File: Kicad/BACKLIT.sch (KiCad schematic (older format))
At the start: 88 parts, among them U1 PAM2804

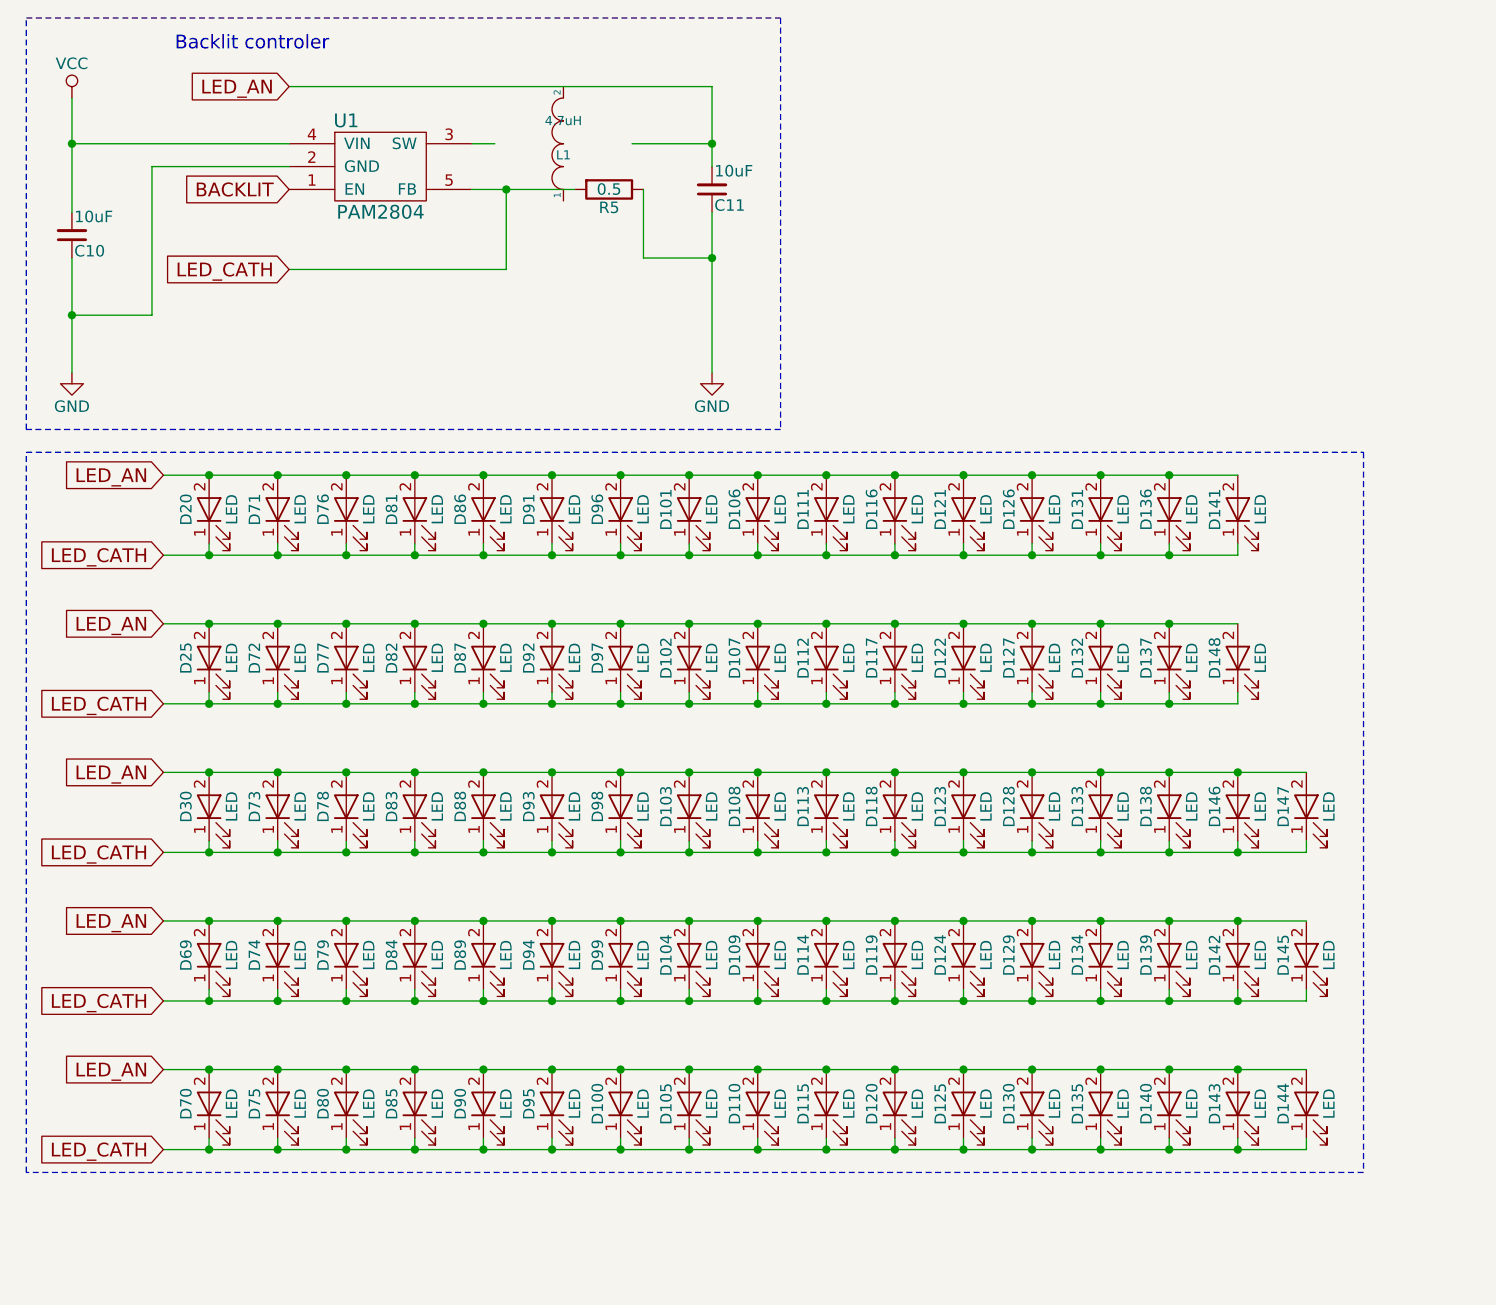
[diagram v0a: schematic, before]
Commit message: - First draw for Rev. B
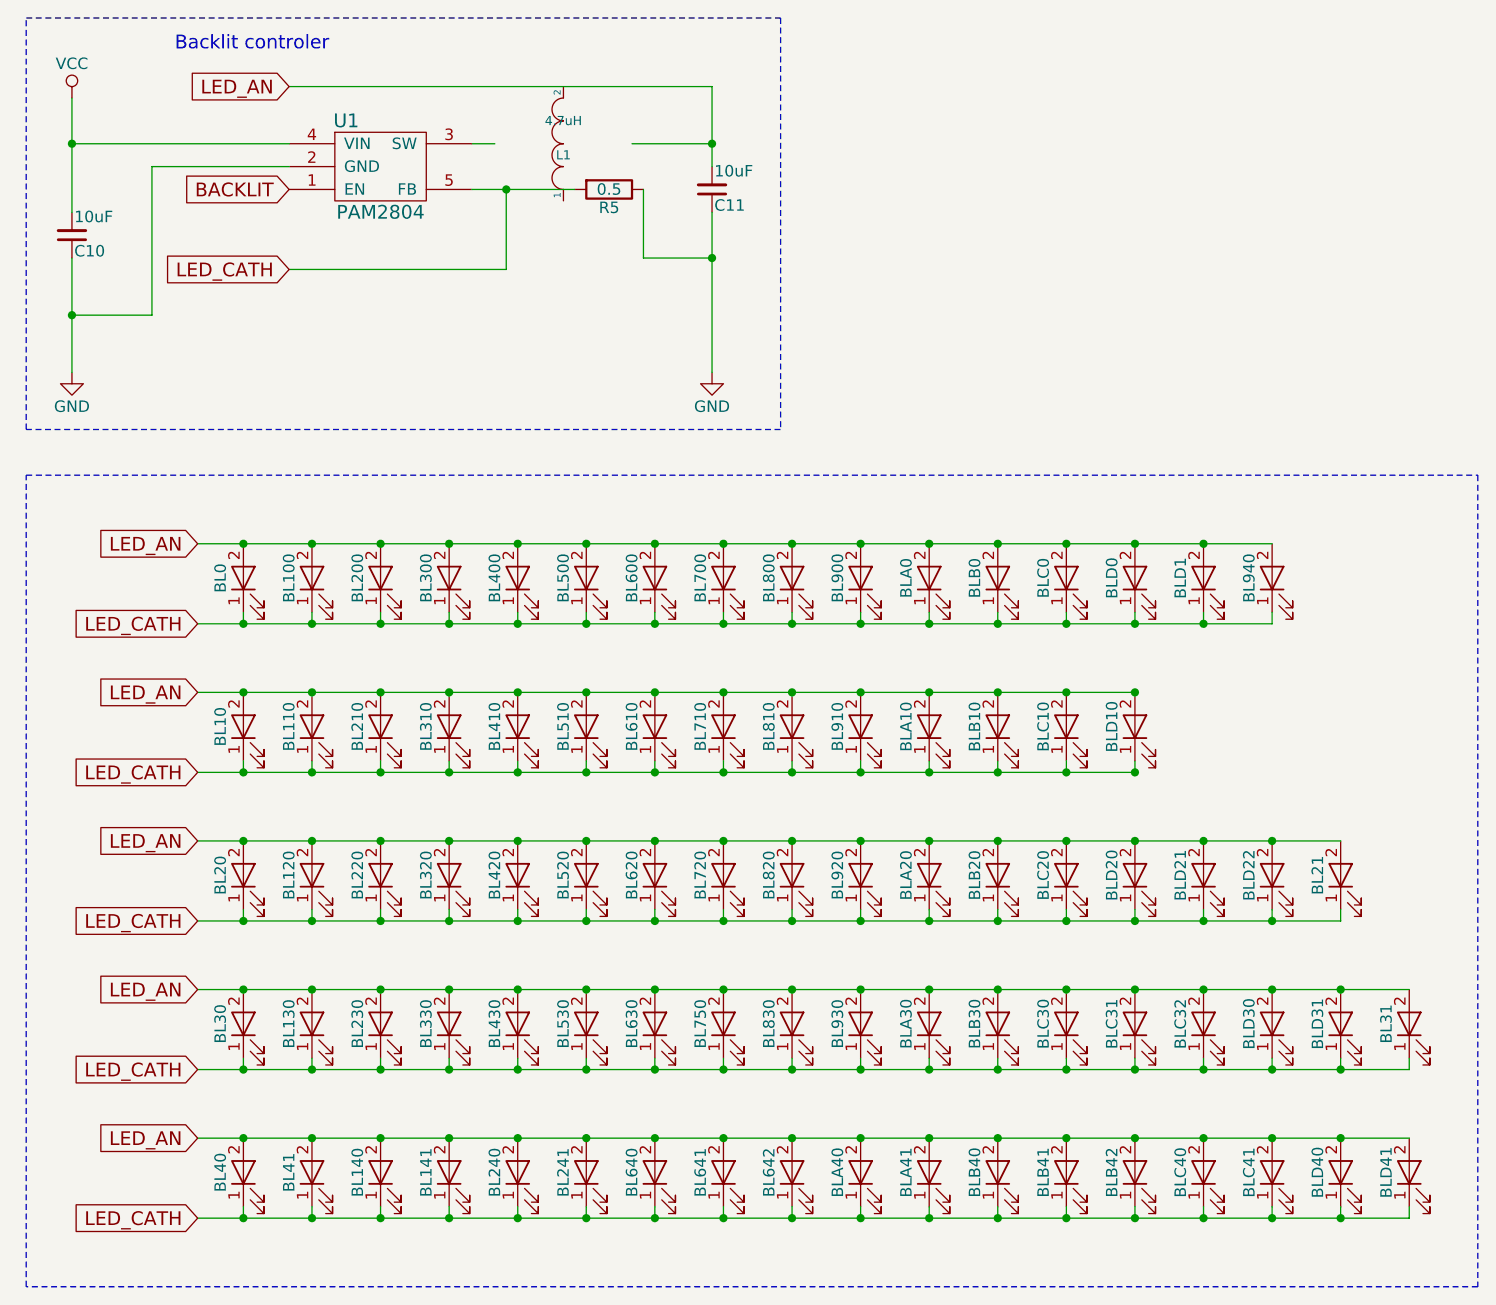
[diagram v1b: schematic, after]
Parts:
- renumbered D20 to BL0, D25 to BL10, D71 to BL100, D72 to BL110, D73 to BL120, D74 to BL130, D80 to BL140, D85 to BL141, D30 to BL20, D76 to BL200, D137 to BL21, D77 to BL210, D78 to BL220, D79 to BL230, D90 to BL240, D95 to BL241, D69 to BL30, D81 to BL300, D148 to BL31, D82 to BL310, D83 to BL320, D84 to BL330, D70 to BL40, D86 to BL400, D75 to BL41, D87 to BL410, D88 to BL420, D89 to BL430, D91 to BL500, D92 to BL510, D93 to BL520, D94 to BL530, D96 to BL600, D97 to BL610, D98 to BL620, D99 to BL630, D100 to BL640, D105 to BL641, D110 to BL642, D101 to BL700, D102 to BL710, D103 to BL720, D104 to BL750, D106 to BL800, D107 to BL810, D108 to BL820, D109 to BL830, D111 to BL900, D112 to BL910, D113 to BL920, D114 to BL930, D141 to BL940, D116 to BLA0, D117 to BLA10, D118 to BLA20, D119 to BLA30, D115 to BLA40, D120 to BLA41, D121 to BLB0, D122 to BLB10, D123 to BLB20, D124 to BLB30, D125 to BLB40, D130 to BLB41, D135 to BLB42, D126 to BLC0, D127 to BLC10, D128 to BLC20, D129 to BLC30, D134 to BLC31, D139 to BLC32, D140 to BLC40, D143 to BLC41, D131 to BLD0, D136 to BLD1, D132 to BLD10, D133 to BLD20, D138 to BLD21, D146 to BLD22, D142 to BLD30, D145 to BLD31, D144 to BLD40, D147 to BLD41
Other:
- moved on the sheet: BL0, BL10, BL100, BL110, BL120, BL130, BL140, BL141, BL20, BL200, BL21, BL210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
